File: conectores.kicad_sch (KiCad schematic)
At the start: 12 parts, among them J10 5v Input, J11 12v Input, J12 Temp DHT22, J2 Fan1 Conn, J3 Fan2 Conn, J4 Fan4 Conn, J5 Fan3 Conn, J6 Buzz Conn, J7 OLED, J8 Relay Ctrl, J9 Relay Out

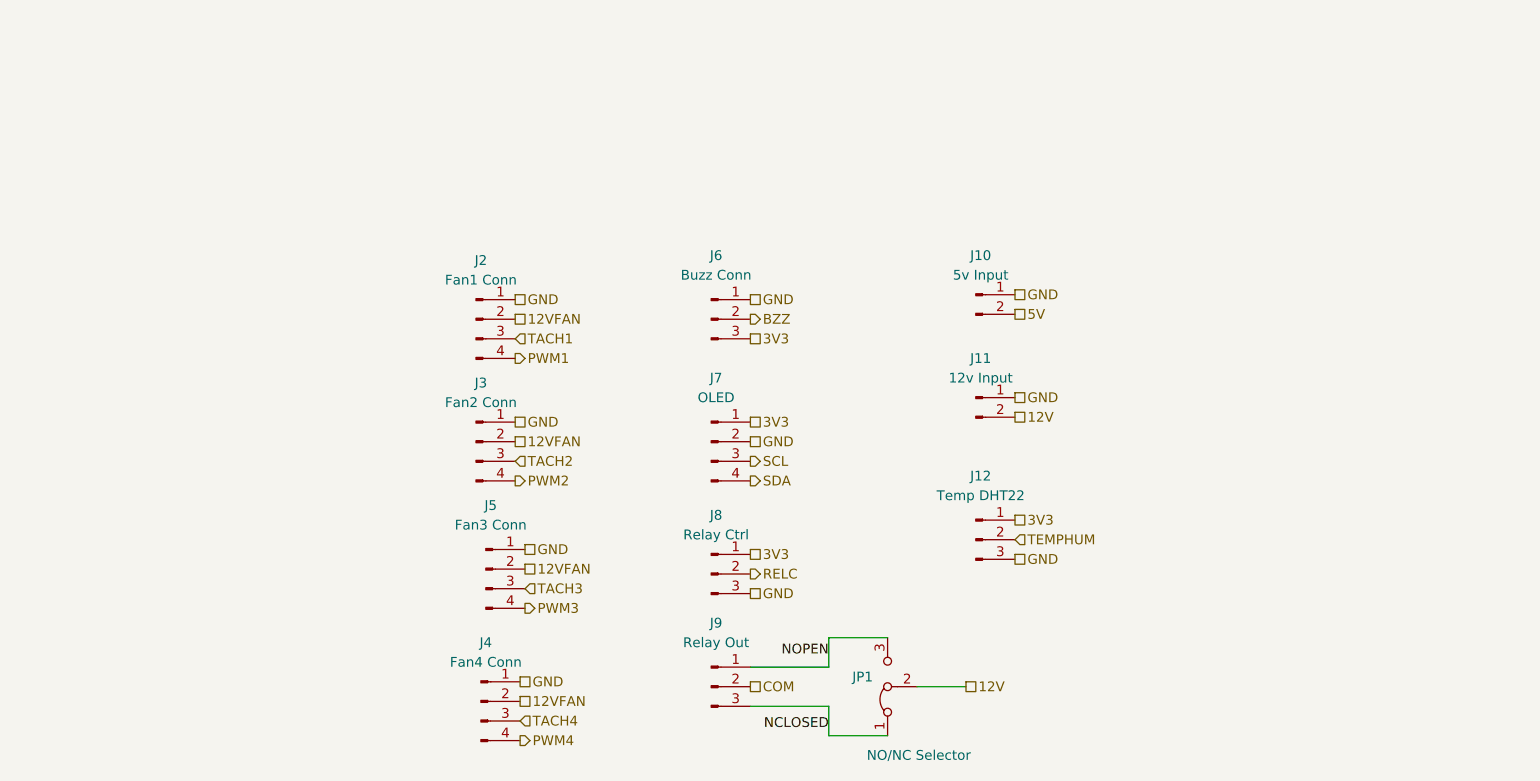
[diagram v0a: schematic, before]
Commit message: pop stashed changes
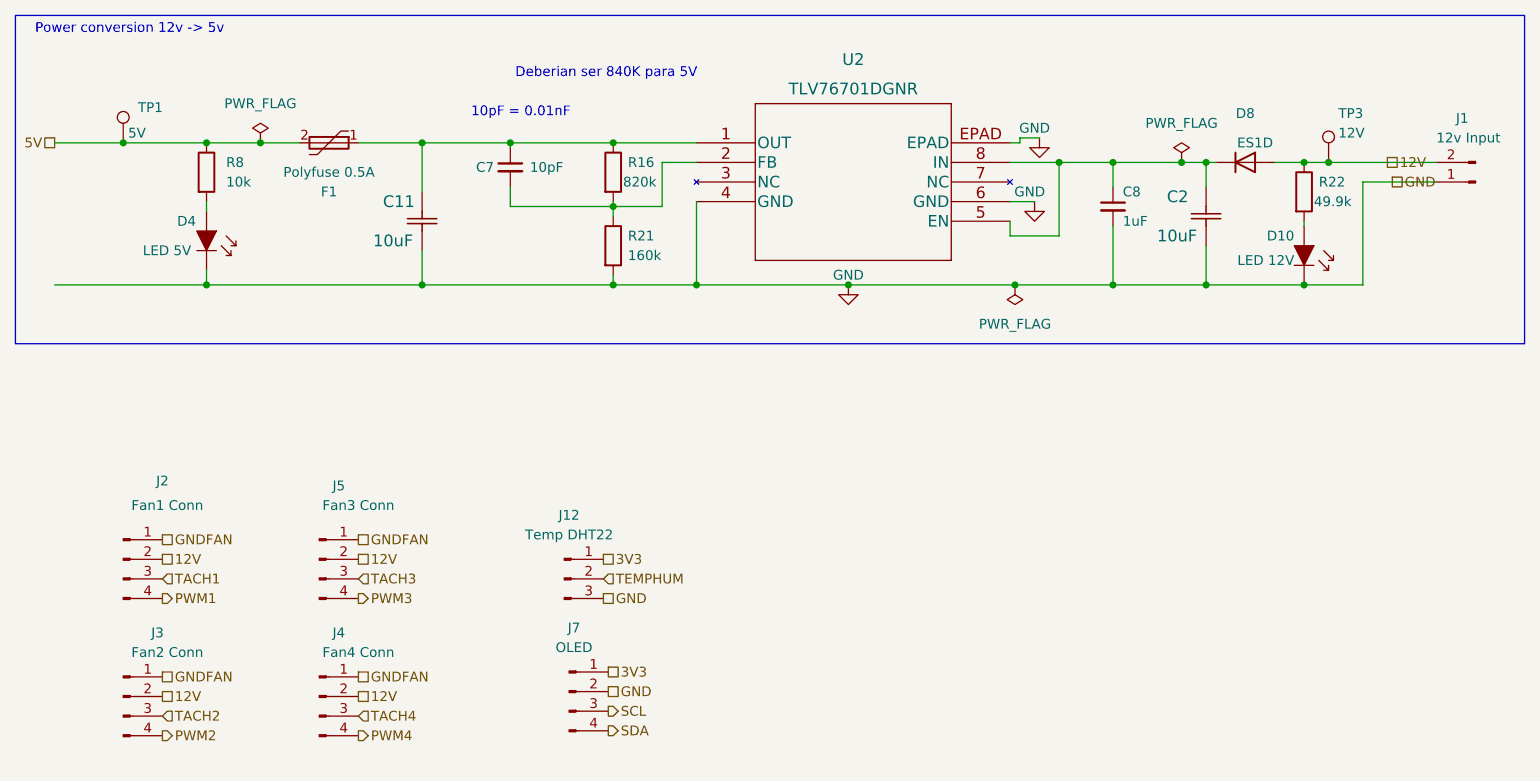
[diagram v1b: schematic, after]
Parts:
- removed J10: 5v Input, Connector_PinHeader_2.54mm:PinHeader_1x02_P2.54mm_Vertical, symbol Connector:Conn_01x02_Male
- removed J11: 12v Input, Connector_PinHeader_2.54mm:PinHeader_1x02_P2.54mm_Vertical, symbol Connector:Conn_01x02_Male
- removed J6: Buzz Conn, Connector_PinHeader_2.54mm:PinHeader_1x03_P2.54mm_Vertical, symbol Connector:Conn_01x03_Male
- removed J8: Relay Ctrl, Connector_PinHeader_2.54mm:PinHeader_1x03_P2.54mm_Vertical, symbol Connector:Conn_01x03_Male
- removed J9: Relay Out, Connector_PinHeader_2.54mm:PinHeader_1x03_P2.54mm_Vertical, symbol Connector:Conn_01x03_Male
- removed JP1: NO/NC Selector, Connector_PinHeader_2.54mm:PinHeader_1x03_P2.54mm_Vertical, symbol Jumper:Jumper_3_Bridged12
- added C11, C2: 10uF, footprints descargados:CL21A106KOQNNNE, symbol CL21A106KOQNNNE:CL21A106KOQNNNE
- added C7: 10pF, Capacitor_SMD:C_0603_1608Metric_Pad1.08x0.95mm_HandSolder, symbol Device:C_Small
- added C8: 1uF, Capacitor_SMD:C_0603_1608Metric_Pad1.08x0.95mm_HandSolder, symbol Device:C_Small
- added D10: LED 12V, digikey-footprints:0805, symbol dk_LED-Indication-Discrete:LG_R971-KN-1
- added D4: LED 5V, digikey-footprints:0805, symbol dk_LED-Indication-Discrete:LG_R971-KN-1
- added D8: ES1D, Diode_SMD:D_1206_3216Metric_Pad1.42x1.75mm_HandSolder, symbol Device:D
- added F1: Polyfuse 0.5A, Fuse:Fuse_1206_3216Metric_Pad1.42x1.75mm_HandSolder, symbol Device:Polyfuse
- added J1: 12v Input, Connector_PinHeader_2.54mm:PinHeader_1x02_P2.54mm_Vertical, symbol Connector:Conn_01x02_Male
- added R16: 820k, Resistor_SMD:R_0603_1608Metric_Pad0.98x0.95mm_HandSolder, symbol Device:R
- added R21: 160k, Resistor_SMD:R_0603_1608Metric_Pad0.98x0.95mm_HandSolder, symbol Device:R
- added R22: 49.9k, Resistor_SMD:R_0603_1608Metric_Pad0.98x0.95mm_HandSolder, symbol Device:R
- added R8: 10k, Resistor_SMD:R_0603_1608Metric_Pad0.98x0.95mm_HandSolder, symbol Device:R
- added TP1: 5V, TestPoint:TestPoint_Pad_D1.5mm, symbol Connector:TestPoint
- added TP3: 12V, TestPoint:TestPoint_Pad_D1.5mm, symbol Connector:TestPoint
- added U2: TLV76701DGNR, footprints descargados:TLV76701DGNR, symbol TLV76701DGNR:TLV76701DGNR
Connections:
- net 12VFAN is gone; now on net 12V: J2.2 (Pin_2), J3.2 (Pin_2), J4.2 (Pin_2), J5.2 (Pin_2)
- net 12V: now also D8.2 (A), J1.2 (Pin_2), R22.1, TP3.1
- net 5V: now also F1.2, R8.1, TP1.1
- net GND: now also C11.2, C2.2, C8.2, D10.2, D4.2, J1.1 (Pin_1), R21.2, U2.4 (GND), U2.6 (GND), U2.EPAD; no longer J2.1 (Pin_1), J3.1 (Pin_1), J4.1 (Pin_1), J5.1 (Pin_1)
- new net: C2.1, C8.1, D8.1 (K), U2.5 (EN), U2.8 (IN)
- new net: C11.1, C7.1, F1.1, R16.1, U2.1 (OUT)
- new net: C7.2, R16.2, R21.1, U2.2 (FB)
- new net: D4.1, R8.2
- new net: D10.1, R22.2
- new net GNDFAN: J2.1 (Pin_1), J3.1 (Pin_1), J4.1 (Pin_1), J5.1 (Pin_1)
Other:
- note added: "10pF = 0.01nF"
- note added: "Deberian ser 840K para 5V"
- note added: "Power conversion 12v -> 5v"
- moved on the sheet: J12, J2, J3, J4, J5, J7
